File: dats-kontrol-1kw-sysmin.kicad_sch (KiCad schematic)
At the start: 2 parts, among them J7 Conn_01x12, U1 YAAJ_WeAct_BlackPill_Part_Lik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

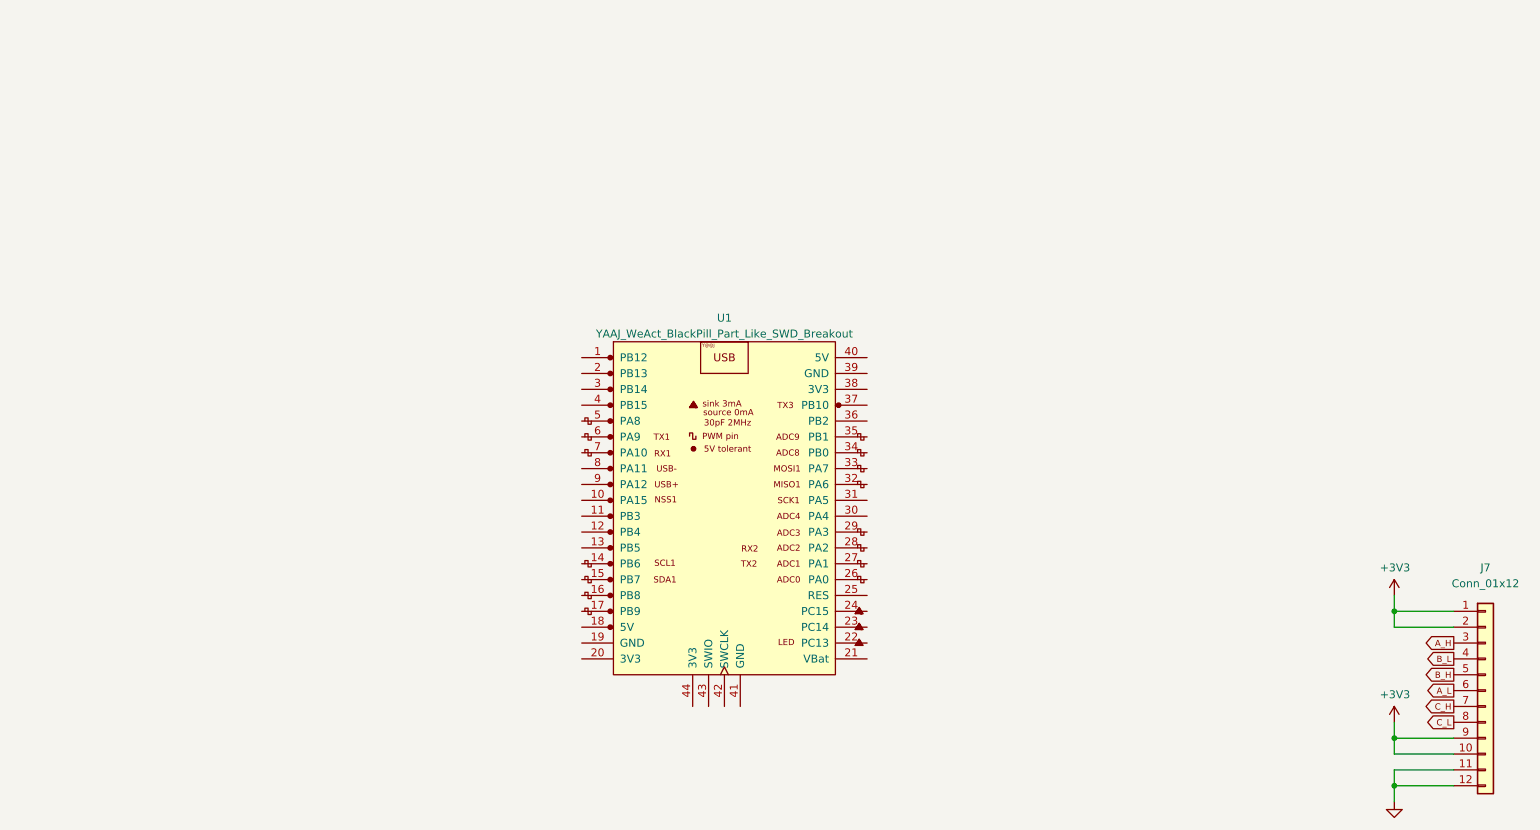
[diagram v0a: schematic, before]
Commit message: Layout STM
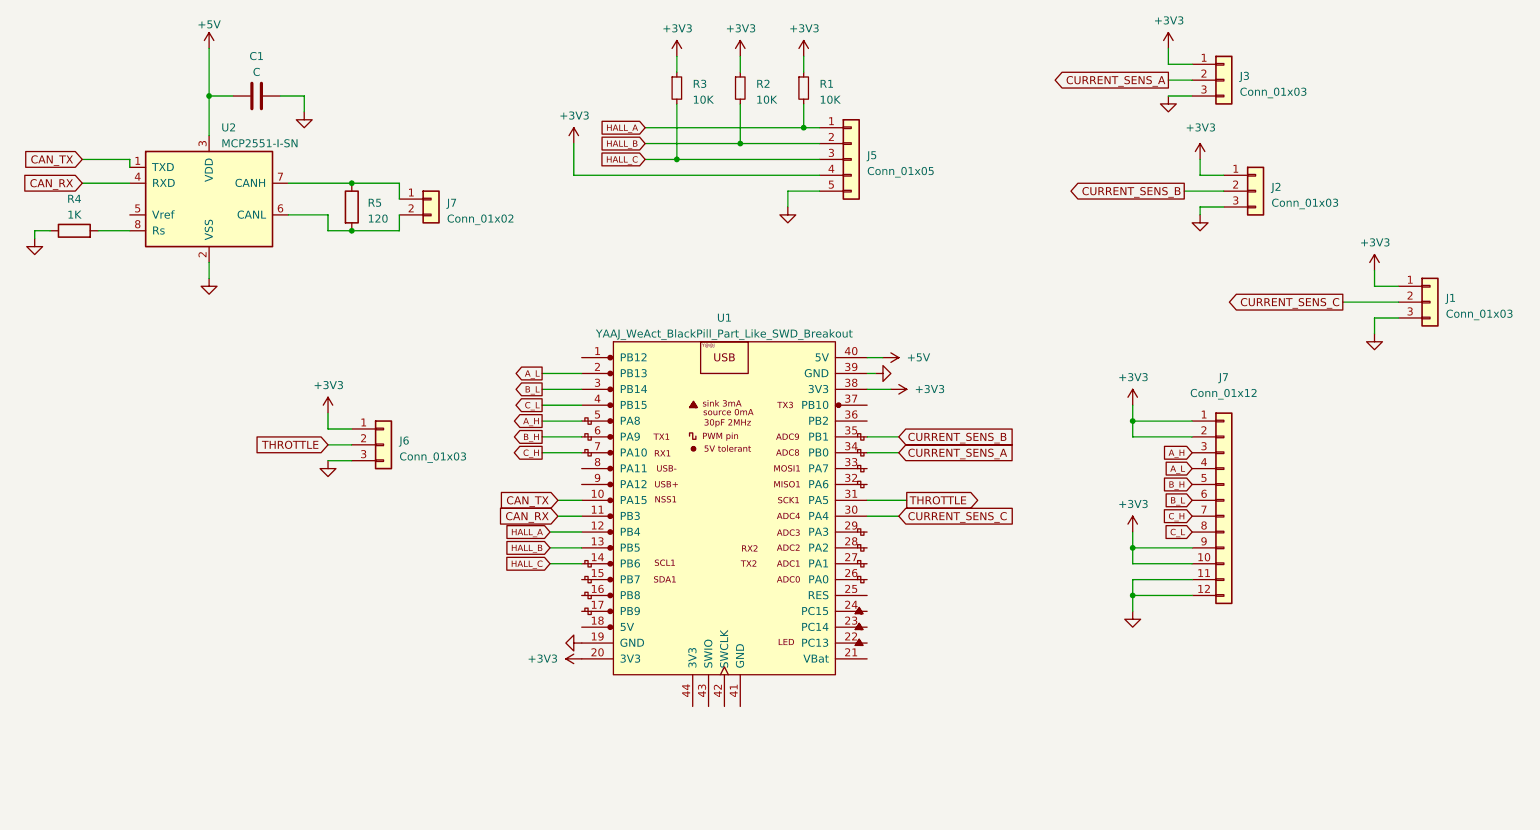
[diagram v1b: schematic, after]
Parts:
- added C1: C, Resistor_SMD:R_0805_2012Metric, symbol Device:C
- added J1, J2, J3: Conn_01x03, Connector_PinHeader_2.54mm:PinHeader_1x03_P2.54mm_Vertical, symbol Connector_Generic:Conn_01x03
- added J5: Conn_01x05, Connector_JST:JST_XH_B5B-XH-A_1x05_P2.50mm_Vertical, symbol Connector_Generic:Conn_01x05
- added J6: Conn_01x03, Connector_JST:JST_XH_B3B-XH-A_1x03_P2.50mm_Vertical, symbol Connector_Generic:Conn_01x03
- added J7: Conn_01x02, Connector_JST:JST_XH_B2B-XH-A_1x02_P2.50mm_Vertical, symbol Connector_Generic:Conn_01x02
- added R1, R2, R3: 10K, Resistor_SMD:R_0805_2012Metric, symbol Device:R_Small
- added R4: 1K, Resistor_SMD:R_0805_2012Metric, symbol Device:R
- added R5: 120, Resistor_SMD:R_0805_2012Metric, symbol Device:R
- added U2: MCP2551-I-SN, Package_SO:SOIC-8_3.9x4.9mm_P1.27mm, symbol Interface_CAN_LIN:MCP2551-I-SN
- J7: footprint Connector_PinHeader_2.54mm:PinHeader_1x12_P2.54mm_Vertical -> Connector_PinHeader_2.54mm:PinHeader_2x06_P2.54mm_Vertical
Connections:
- net +3V3: now also U1.20 (3V3), U1.38 (3V3), J1.1 (Pin_1), J2.1 (Pin_1), J3.1 (Pin_1), J5.4 (Pin_4), J6.1 (Pin_1), R1.1, R2.1, R3.1
- net A_H: now also U1.5 (PA8)
- net A_L: now also J7.4 (Pin_4), U1.2 (PB13); no longer J7.6 (Pin_6)
- net B_H: now also U1.6 (PA9)
- net B_L: now also J7.6 (Pin_6), U1.3 (PB14); no longer J7.4 (Pin_4)
- net C_H: now also U1.7 (PA10)
- net C_L: now also U1.4 (PB15)
- net GND: now also U1.19 (GND), U1.39 (GND), C1.2, J1.3 (Pin_3), J2.3 (Pin_3), J3.3 (Pin_3), J5.5 (Pin_5), J6.3 (Pin_3), R4.1, U2.2 (VSS)
- net CAN_TX: now reaches U1.10 (PA15)
- net CAN_TX: now also U2.1 (TXD)
- net CAN_RX: now reaches U1.11 (PB3)
- net CAN_RX: now also U2.4 (RXD)
- net HALL_A: now reaches U1.12 (PB4)
- net HALL_A: now also J5.1 (Pin_1), R1.2
- net HALL_B: now reaches U1.13 (PB5)
- net HALL_B: now also J5.2 (Pin_2), R2.2
- net HALL_C: now reaches U1.14 (PB6)
- net HALL_C: now also J5.3 (Pin_3), R3.2
- net CURRENT_SENS_C: now reaches U1.30 (PA4)
- net CURRENT_SENS_C: now also J1.2 (Pin_2)
- net THROTTLE: now reaches U1.31 (PA5)
- net THROTTLE: now also J6.2 (Pin_2)
- net CURRENT_SENS_A: now reaches U1.34 (PB0)
- net CURRENT_SENS_A: now also J3.2 (Pin_2)
- net CURRENT_SENS_B: now reaches U1.35 (PB1)
- net CURRENT_SENS_B: now also J2.2 (Pin_2)
- net +5V: now reaches U1.40 (5V)
- net +5V: now also C1.1, U2.3 (VDD)
- new net: J7.2 (Pin_2), R5.2, U2.6 (CANL)
- new net: J7.1 (Pin_1), R5.1, U2.7 (CANH)
- new net: R4.2, U2.8 (Rs)
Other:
- moved on the sheet: J7
